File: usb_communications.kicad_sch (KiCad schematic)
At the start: 46 parts, among them J1 USB_C, J2 CAN, J6 UART, Q10 2N7002, Q3 2N7002, Q6 BS138, Q7 BS138, U2 TPD2E2U06, U3 MCP2518FD, U4 MCP2562FD, Y1 20Mhz

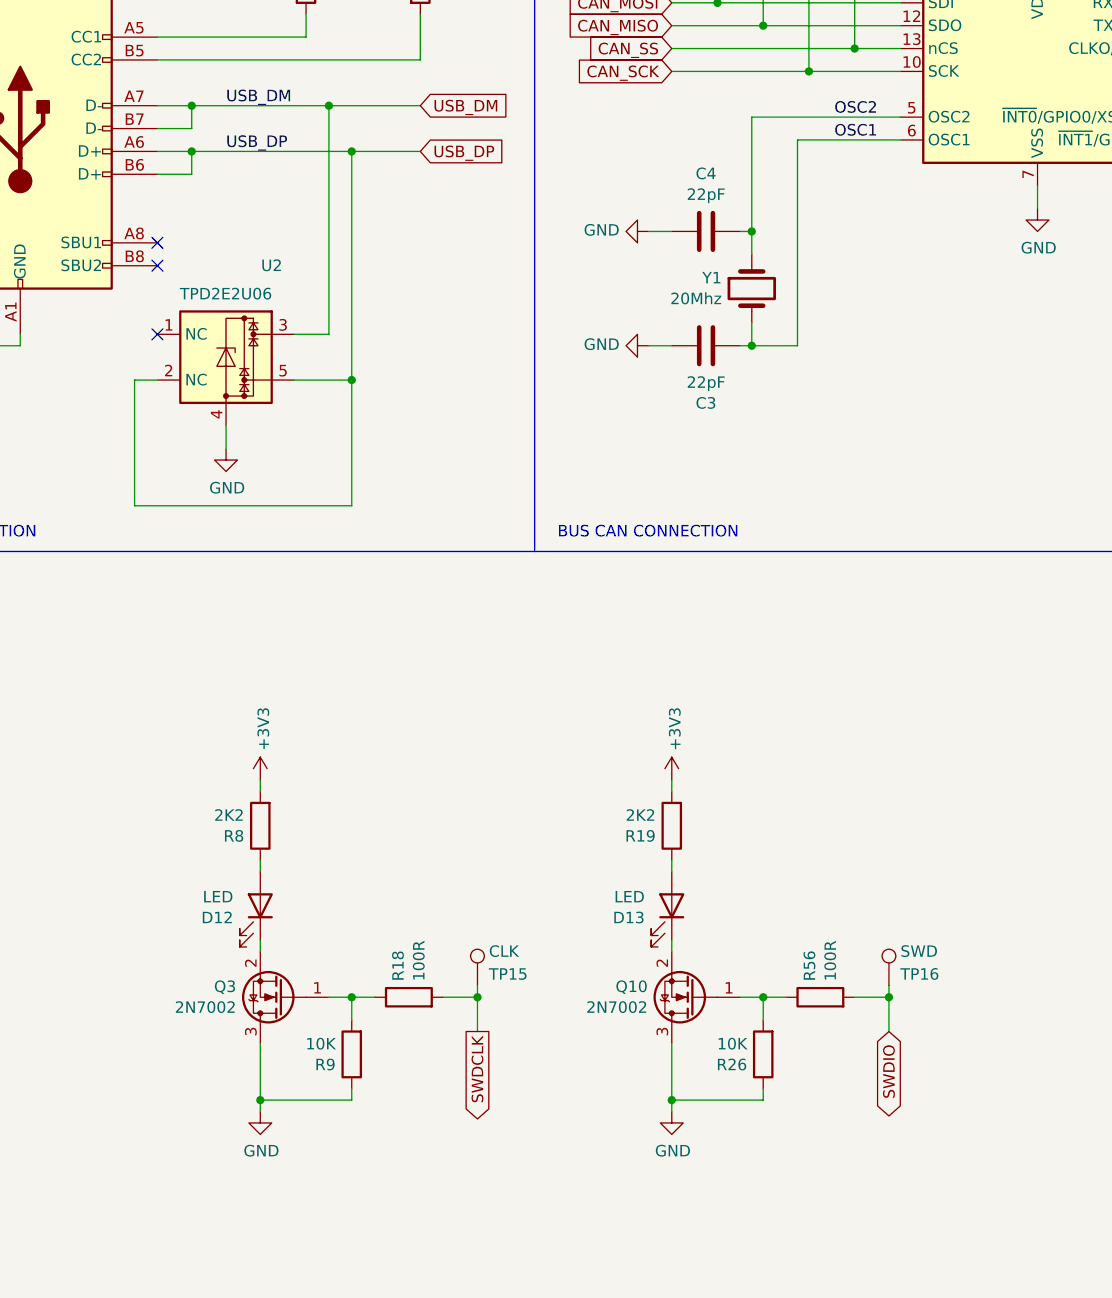
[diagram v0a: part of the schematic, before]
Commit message: 25/01/24/A
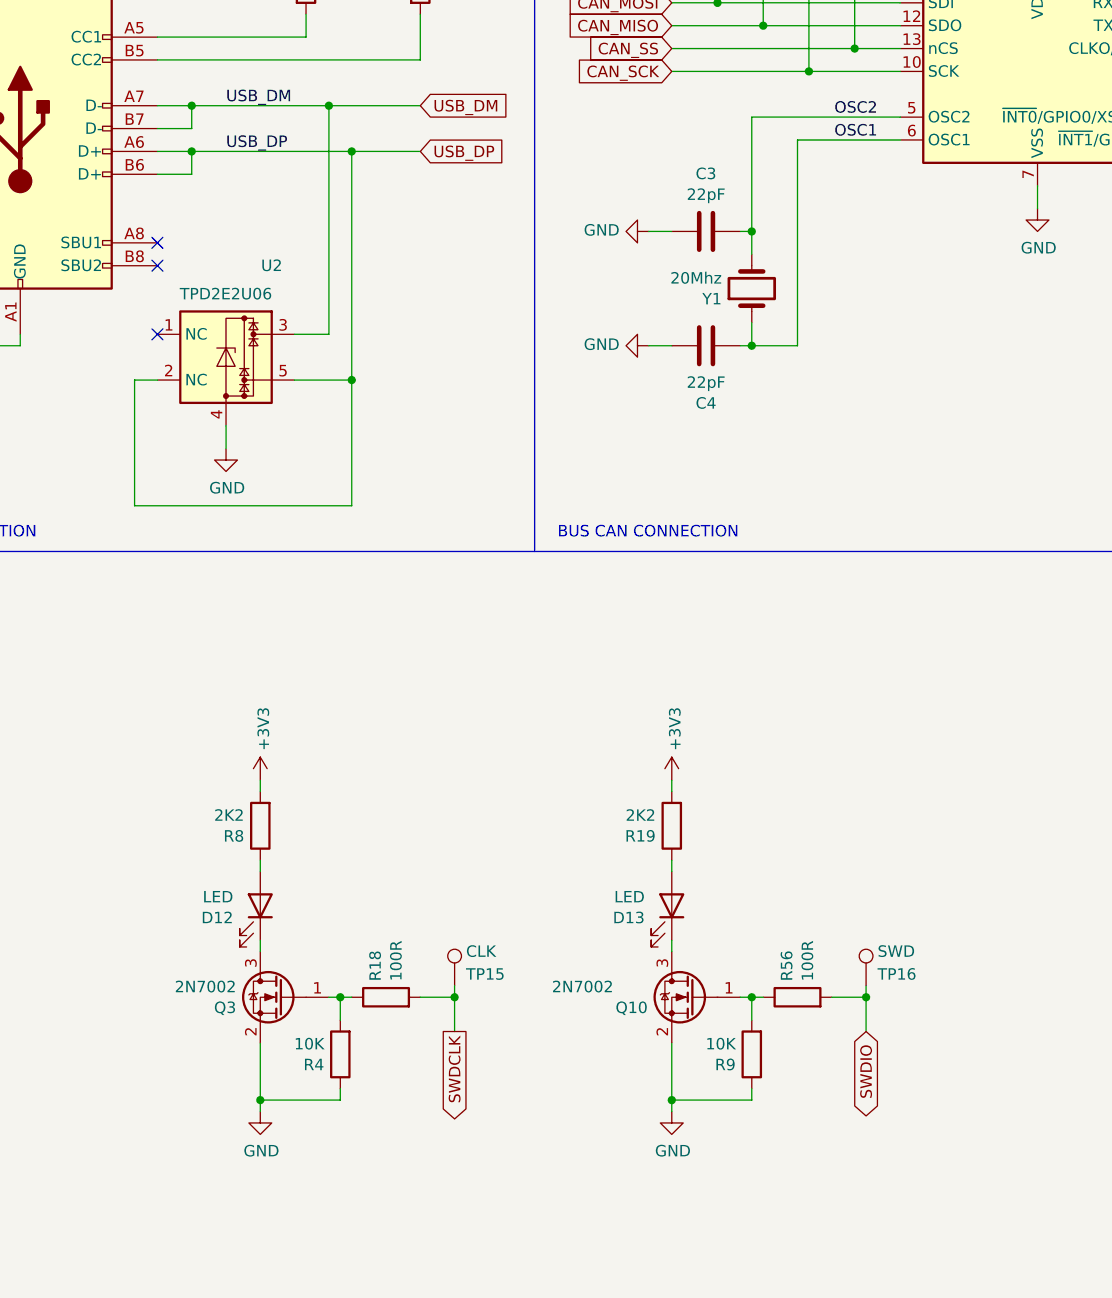
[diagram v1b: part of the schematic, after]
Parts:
- removed R26: 10K, Resistor_SMD:R_1206_3216Metric, symbol Device:R
- added R4: 10K, Resistor_SMD:R_1206_3216Metric, symbol Device:R
- F1: footprint x_Fuses:MF-SMDF200-2 -> x_Fuses:MF_SMDF200
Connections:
- net GND: now also Q10.2 (S), Q3.2 (S), R4.1; no longer Q10.3 (D), Q3.3 (D)
- net OSC1: now also C4.2, Y1.1; no longer C3.2, Y1.2
- net OSC2: now also C3.2, Y1.2; no longer C4.2, Y1.1
- net at Q3.1 (G), R18.1: now also R4.2; no longer R9.2
- net at D12.1 (K): now also Q3.3 (D); no longer Q3.2 (S)
- net at Q10.1 (G), R56.1: now also R9.2
- net at D13.1 (K): now also Q10.3 (D); no longer Q10.2 (S)
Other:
- moved on the sheet: C3, C4, Q10, Q3, R18, R56, TP15, TP16

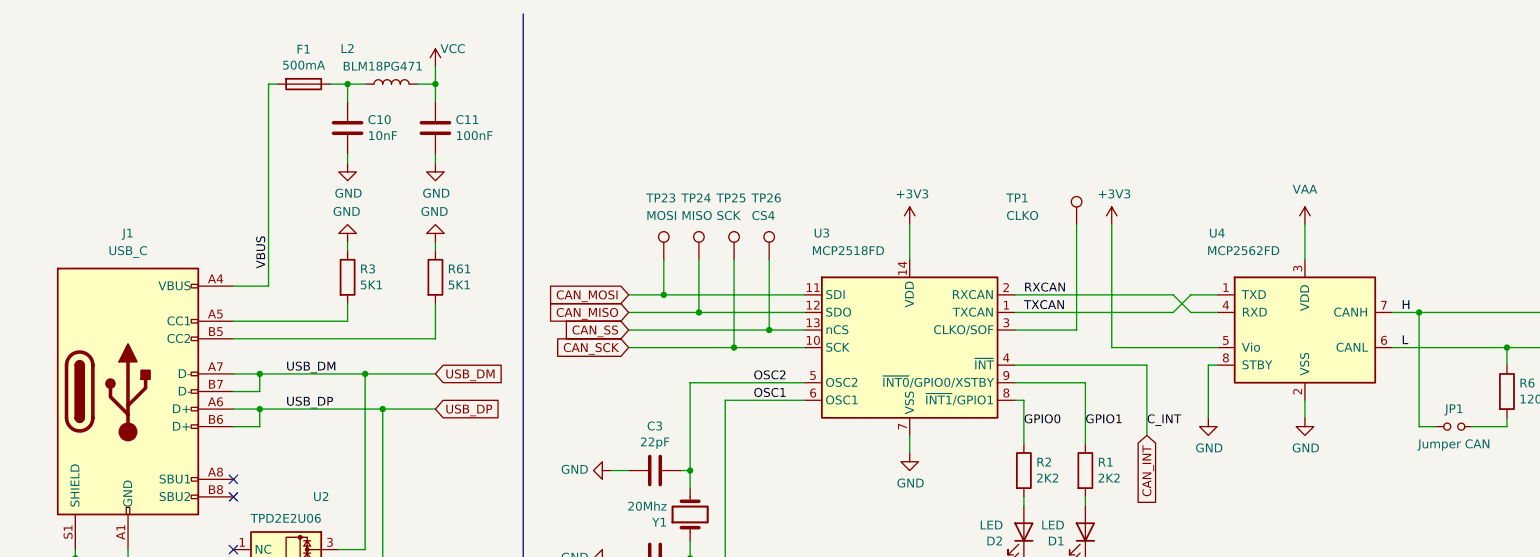
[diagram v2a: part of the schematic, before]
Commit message: 05/25/25/A
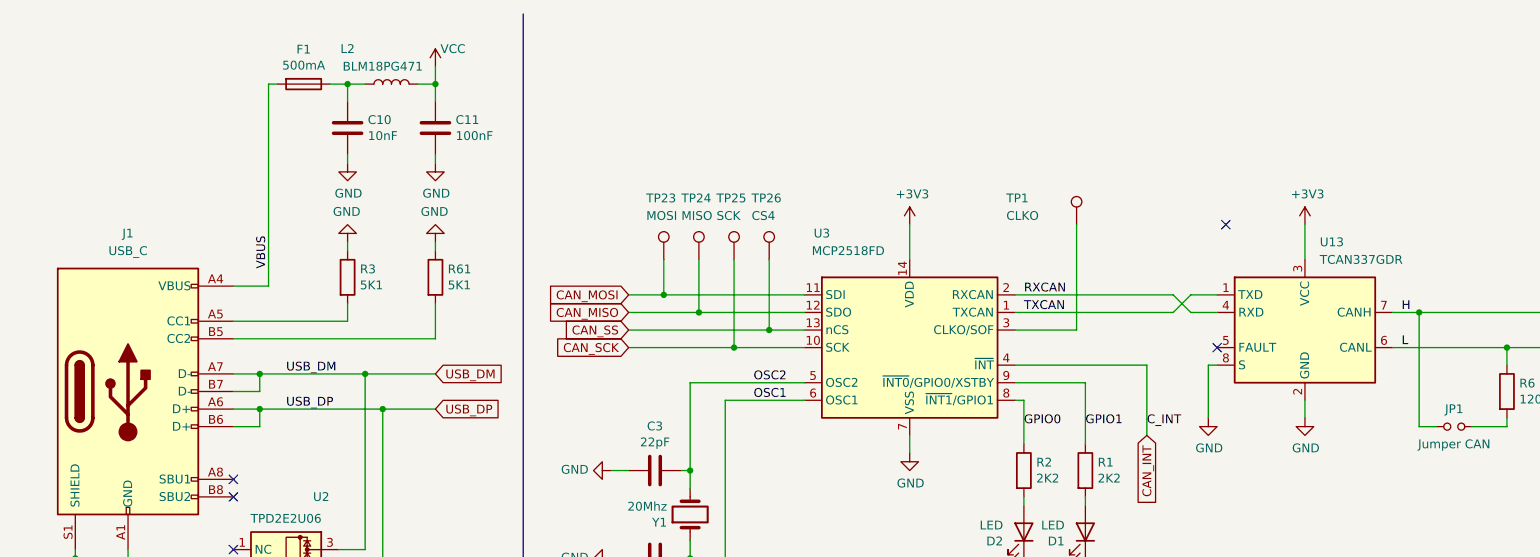
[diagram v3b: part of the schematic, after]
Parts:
- removed U4: MCP2562FD, Package_SO:SOIC-8_3.9x4.9mm_P1.27mm, symbol Interface_CAN_LIN:MCP2562-E-SN
- added U13: TCAN337GDR, Package_SO:SOIC-8_3.9x4.9mm_P1.27mm, symbol Interface_CAN_LIN:TCAN337G
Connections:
- net +3V3: now also U13.3 (VCC)
- net GND: now also U13.2 (GND), U13.8 (S)
- net H: now also U13.7 (CANH)
- net L: now also U13.6 (CANL)
- net RXCAN: now also U13.4 (RXD)
- net TXCAN: now also U13.1 (TXD)
- no-connect marks 3 -> 5
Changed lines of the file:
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@@
 (kicad_sch
-	(version 20231120)
+	(version 20250114)
 	(generator "eeschema")
-	(generator_version "8.0")
+	(generator_version "9.0")
 	(paper "USLetter")
 	(title_block
@@
 		(rev "R4")
 	)
+	(text "BUS CAN CONNECTION"
+		(exclude_from_sim no)
+		(at 87.63 113.03 0)
+		(effects
+			(font
+				(size 1.27 1.27)
+			)
+			(justify left bottom)
+		)
+	)
+	(text "STATUS LEDS"
+		(exclude_from_sim no)
+		(at 13.97 201.93 0)
+		(effects
+			(font
+				(size 1.27 1.27)
+			)
+			(justify left bottom)
+		)
+	)
+	(text "USB CONECCTION"
+		(exclude_from_sim no)
+		(at 13.97 113.03 0)
+		(effects
+			(font
+				(size 1.27 1.27)
+			)
+			(justify left bottom)
+		)
+	)
 	(junction
 		(at 76.2 163.83)
@@
 	)
 	(no_connect
+		(at 185.42 60.96)
+	)
+	(no_connect
+		(at 186.69 43.18)
+	)
+	(no_connect
 		(at 43.18 80.01)
 	)
@@
 	(wire
 		(pts
-			(xy 170.18 60.96) (xy 185.42 60.96)
-		)
-		(stroke
-			(width 0)
-			(type default)
-		)
-	)
-	(wire
-		(pts
 			(xy 207.01 124.46) (xy 241.3 124.46)
 		)
@@
 	(wire
 		(pts
-			(xy 170.18 43.18) (xy 170.18 60.96)
-		)
-		(stroke
-			(width 0)
-			(type default)
-		)
-	)
-	(wire
-		(pts
 			(xy 72.39 20.32) (xy 72.39 22.86)
 		)
@@
 		)
 	)
-	(text "BUS CAN CONNECTION"
-		(exclude_from_sim no)
-		(at 87.63 113.03 0)
-		(effects
-			(font
-				(size 1.27 1.27)
-			)
-			(justify left bottom)
-		)
-	)
-	(text "STATUS LEDS"
-		(exclude_from_sim no)
-		(at 13.97 201.93 0)
-		(effects
-			(font
-				(size 1.27 1.27)
-			)
-			(justify left bottom)
-		)
-	)
-	(text "USB CONECCTION"
-		(exclude_from_sim no)
-		(at 13.97 113.03 0)
-		(effects
-			(font
-				(size 1.27 1.27)
-			)
-			(justify left bottom)
-		)
-	)
 	(label "OSC2"
 		(at 123.19 66.04 180)
@@
 	)
 	(symbol
-		(lib_id "Interface_CAN_LIN:MCP2562-E-SN")
-		(at 198.12 58.42 0)
-		(unit 1)
-		(exclude_from_sim no)
-		(in_bom yes)
-		(on_board yes)
-		(dnp no)
-		(property "Reference" "U4"
-			(at 185.42 44.45 0)
-			(effects
-				(font
-					(size 1.27 1.27)
-				)
-			)
-		)
-		(property "Value" "MCP2562FD"
-			(at 189.23 46.99 0)
-			(effects
-				(font
-					(size 1.27 1.27)
-				)
-			)
-		)
-		(property "Footprint" "Package_SO:SOIC-8_3.9x4.9mm_P1.27mm"
-			(at 198.12 71.12 0)
-			(effects
-				(font
-					(size 1.27 1.27)
-					(italic yes)
-				)
-				(hide yes)
-			)
-		)
-		(property "Datasheet" "http://ww1.microchip.com/downloads/en/DeviceDoc/25167A.pdf"
-			(at 198.12 58.42 0)
-			(effects
-				(font
-					(size 1.27 1.27)
-				)
-				(hide yes)
-			)
-		)
-		(property "Description" ""
-			(at 198.12 58.42 0)
-			(effects
-				(font
-					(size 1.27 1.27)
-				)
-				(hide yes)
-			)
-		)
-		(pin "1"
-		)
-		(pin "2"
-		)
-		(pin "3"
-		)
-		(pin "4"
-		)
-		(pin "5"
-		)
-		(pin "6"
-		)
-		(pin "7"
-		)
-		(pin "8"
-		)
-		(instances
-			(project "Game_Cat_R4"
-				(path "/96315415-cfed-47d2-b3dd-d782358bd0df/00000000-0000-0000-0000-00005cbab8ae"
-					(reference "U4")
-					(unit 1)
-				)
-			)
-		)
-	)
-	(symbol
 		(lib_id "Device:Jumper_NO_Small")
 		(at 219.71 72.39 0)
@@
 	)
 	(symbol
-		(lib_id "power:+3.3V")
-		(at 170.18 43.18 0)
-		(unit 1)
-		(exclude_from_sim no)
-		(in_bom yes)
-		(on_board yes)
-		(dnp no)
-		(property "Reference" "#PWR015"
-			(at 170.18 46.99 0)
-			(effects
-				(font
-					(size 1.27 1.27)
-				)
-				(hide yes)
-			)
-		)
-		(property "Value" "+3V3"
-			(at 170.561 38.7858 0)
-			(effects
-				(font
-					(size 1.27 1.27)
-				)
-			)
-		)
-		(property "Footprint" ""
-			(at 170.18 43.18 0)
-			(effects
-				(font
-					(size 1.27 1.27)
-				)
-				(hide yes)
-			)
-		)
-		(property "Datasheet" ""
-			(at 170.18 43.18 0)
-			(effects
-				(font
-					(size 1.27 1.27)
-				)
-				(hide yes)
-			)
-		)
-		(property "Description" ""
-			(at 170.18 43.18 0)
-			(effects
-				(font
-					(size 1.27 1.27)
-				)
-				(hide yes)
-			)
-		)
-		(pin "1"
-		)
-		(instances
-			(project "Game_Cat_R4"
-				(path "/96315415-cfed-47d2-b3dd-d782358bd0df/00000000-0000-0000-0000-00005cbab8ae"
-					(reference "#PWR015")
-					(unit 1)
-				)
-			)
-		)
-	)
-	(symbol
 		(lib_id "Device:LED")
 		(at 157.48 87.63 270)
@@
 	)
 	(symbol
+		(lib_id "power:+3.3V")
+		(at 198.12 43.18 0)
+		(unit 1)
+		(exclude_from_sim no)
+		(in_bom yes)
+		(on_board yes)
+		(dnp no)
+		(property "Reference" "#PWR013"
+			(at 198.12 46.99 0)
+			(effects
+				(font
+					(size 1.27 1.27)
+				)
+				(hide yes)
+			)
+		)
+		(property "Value" "+3V3"
+			(at 198.501 38.7858 0)
+			(effects
+				(font
+					(size 1.27 1.27)
+				)
+			)
+		)
+		(property "Footprint" ""
+			(at 198.12 43.18 0)
+			(effects
+				(font
+					(size 1.27 1.27)
+				)
+				(hide yes)
+			)
+		)
+		(property "Datasheet" ""
+			(at 198.12 43.18 0)
+			(effects
+				(font
+					(size 1.27 1.27)
+				)
+				(hide yes)
+			)
+		)
+		(property "Description" ""
+			(at 198.12 43.18 0)
+			(effects
+				(font
+					(size 1.27 1.27)
+				)
+				(hide yes)
+			)
+		)
+		(pin "1"
+		)
+		(instances
+			(project "Game_Cat_R4"
+				(path "/96315415-cfed-47d2-b3dd-d782358bd0df/00000000-0000-0000-0000-00005cbab8ae"
+					(reference "#PWR013")
+					(unit 1)
+				)
+			)
+		)
+	)
+	(symbol
 		(lib_id "Connector:TestPoint")
 		(at 120.65 48.26 0)
@@
 	)
 	(symbol
-		(lib_id "power:VAA")
-		(at 198.12 43.18 0)
+		(lib_id "Interface_CAN_LIN:TCAN337G")
+		(at 198.12 58.42 0)
 		(unit 1)
 		(exclude_from_sim no)
@@
 		(dnp no)
 		(fields_autoplaced yes)
-		(property "Reference" "#PWR0154"
-			(at 198.12 46.99 0)
+		(property "Reference" "U13"
+			(at 200.2633 45.72 0)
 			(effects
 				(font
 					(size 1.27 1.27)
 				)
-				(hide yes)
+				(justify left)
 			)
 		)
-		(property "Value" "VAA"
-			(at 198.12 38.1 0)
+		(property "Value" "TCAN337GDR"
+			(at 200.2633 48.26 0)
 			(effects
 				(font
 					(size 1.27 1.27)
 				)
+				(justify left)
 			)
 		)
-		(property "Footprint" ""
-			(at 198.12 43.18 0)
+		(property "Footprint" "Package_SO:SOIC-8_3.9x4.9mm_P1.27mm"
+			(at 198.12 71.12 0)
 			(effects
 				(font
 					(size 1.27 1.27)
+					(italic yes)
 				)
 				(hide yes)
 			)
 		)
-		(property "Datasheet" ""
-			(at 198.12 43.18 0)
+		(property "Datasheet" "http://www.ti.com/lit/ds/symlink/tcan337.pdf"
+			(at 198.12 58.42 0)
 			(effects
 				(font
@@
 			)
 		)
-		(property "Description" ""
-			(at 198.12 43.18 0)
+		(property "Description" "High-Speed CAN Transceiver with CAN FD, 5Mbps, 3.3V supply, silent mode, fault output, SOT-23-8/SOIC-8"
+			(at 198.12 58.42 0)
 			(effects
 				(font
@@
 			)
 		)
+		(pin "6"
+		)
+		(pin "2"
+		)
+		(pin "7"
+		)
+		(pin "8"
+		)
+		(pin "3"
+		)
+		(pin "5"
+		)
+		(pin "4"
+		)
 		(pin "1"
 		)
 		(instances
-			(project "Game_Cat_R4"
+			(project ""
 				(path "/96315415-cfed-47d2-b3dd-d782358bd0df/00000000-0000-0000-0000-00005cbab8ae"
-					(reference "#PWR0154")
+					(reference "U13")
 					(unit 1)
 				)
